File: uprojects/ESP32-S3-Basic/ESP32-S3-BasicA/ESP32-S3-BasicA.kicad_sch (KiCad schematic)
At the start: 5 parts, among them U1 ESP32-S3-WROOM-1x-N8R8

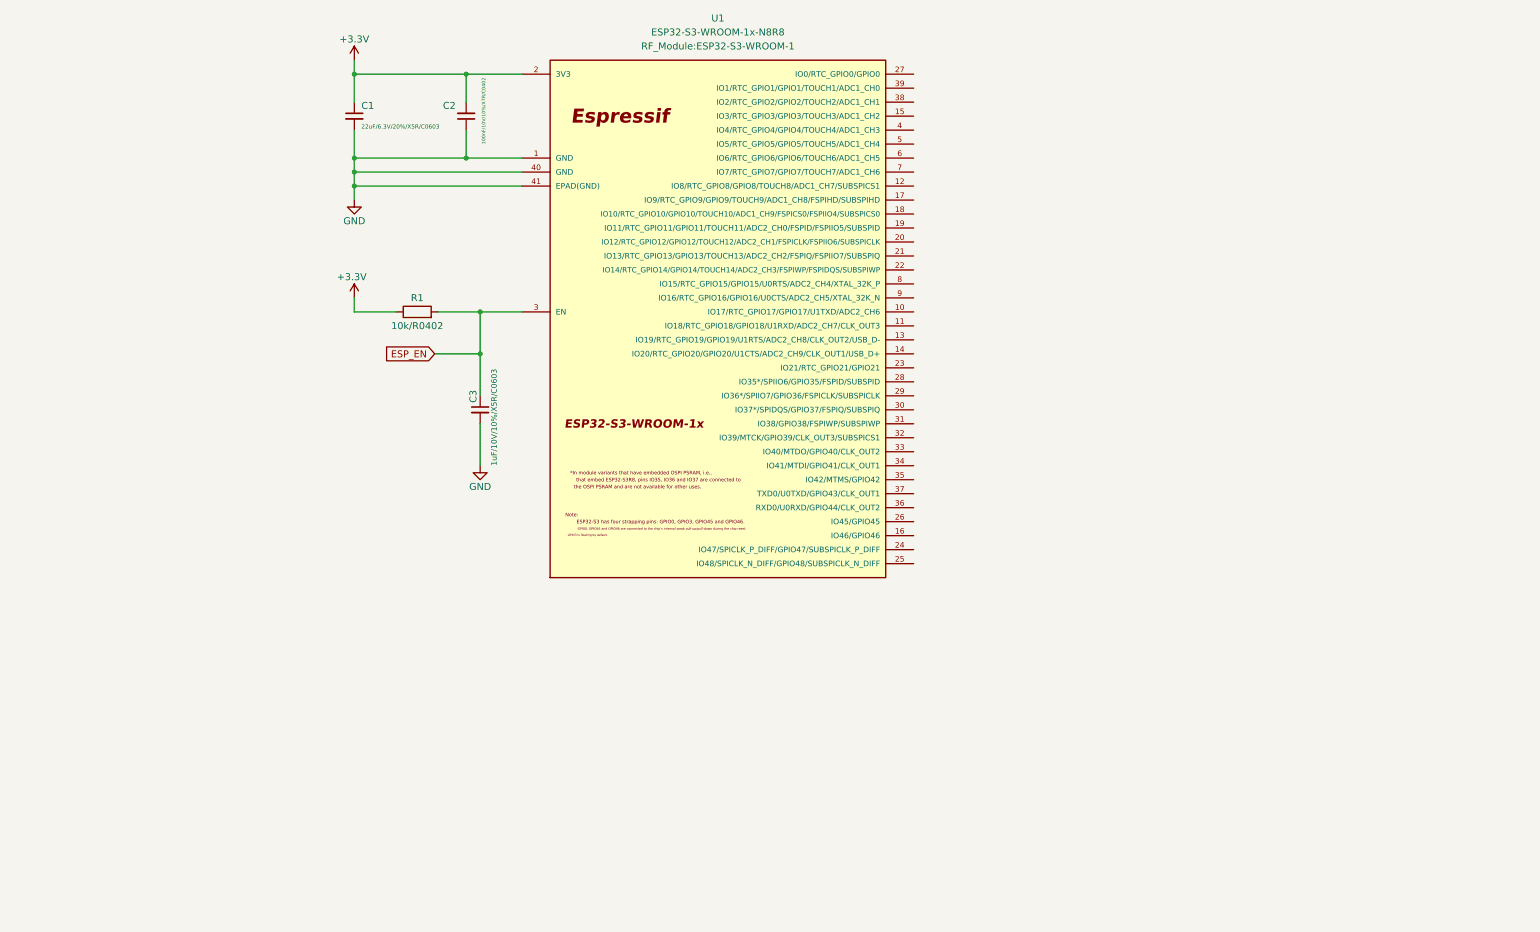
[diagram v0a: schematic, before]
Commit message: April 1 commit
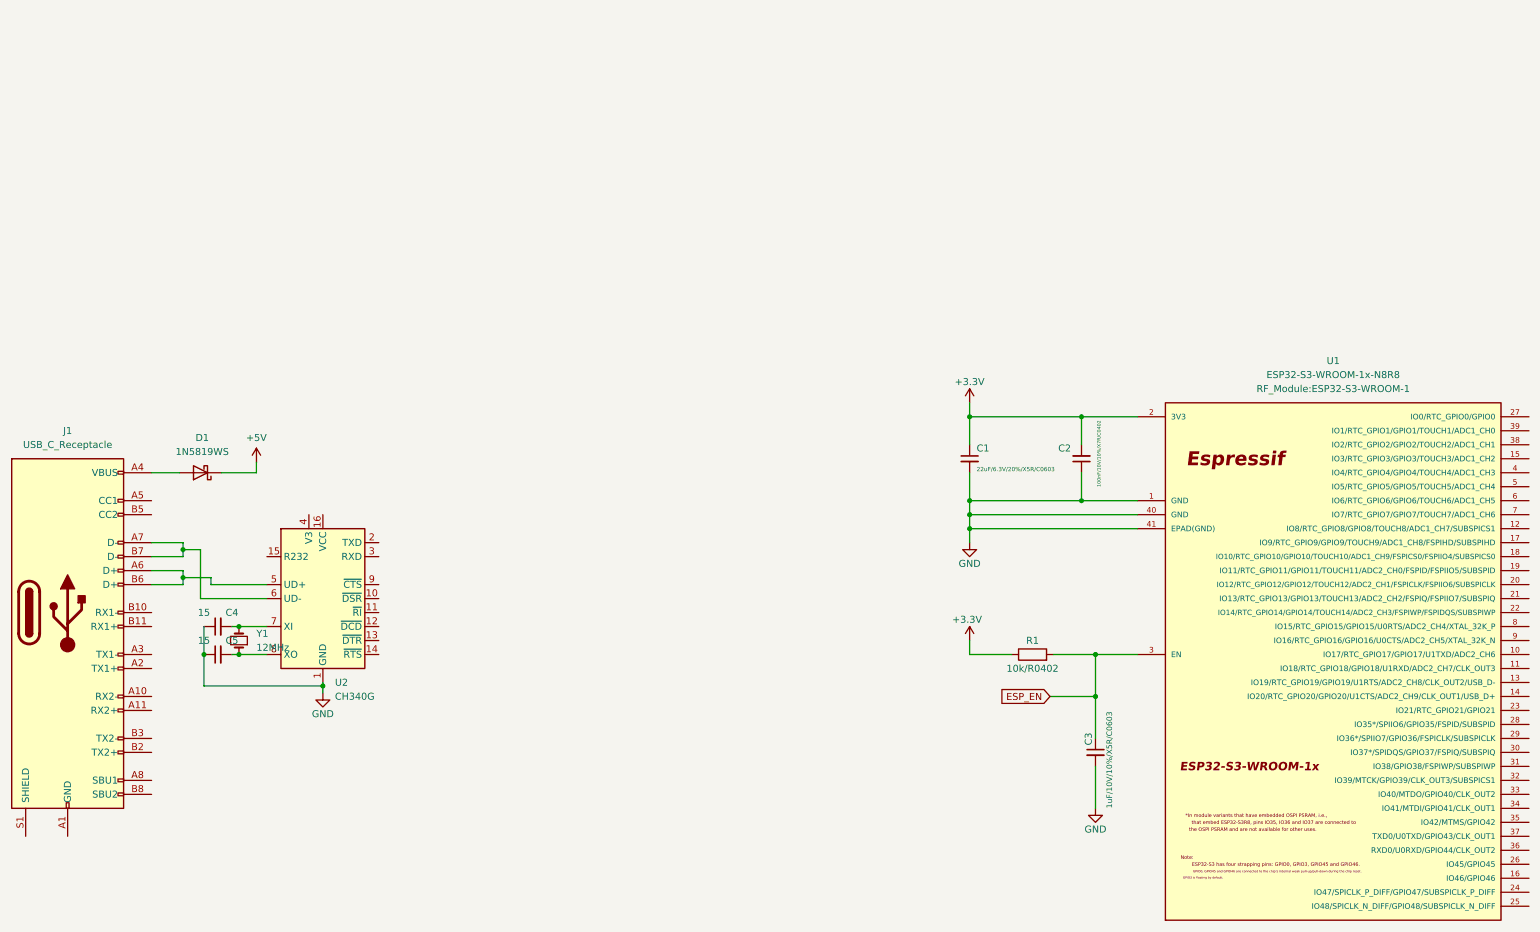
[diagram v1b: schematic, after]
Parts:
- added C4, C5: 15, Capacitor_SMD:C_0805_2012Metric_Pad1.18x1.45mm_HandSolder, symbol Device:C_Small
- added D1: 1N5819WS, Diode_SMD:D_SOD-323, symbol Diode:1N5819WS
- added J1: USB_C_Receptacle, Connector_USB:USB_C_Receptacle_Amphenol_12401610E4-2A_CircularHoles, symbol Connector:USB_C_Receptacle
- added U2: CH340G, Package_SO:SOIC-16_3.9x9.9mm_P1.27mm, symbol Interface_USB:CH340G
- added Y1: 12MHz, Crystal:Crystal_HC49-U_Vertical, symbol Device:Crystal_Small
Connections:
- net GND: now also C4.1, C5.1, U2.1 (GND)
- new net: C5.2, U2.8 (XO), Y1.1
- new net: C4.2, U2.7 (XI), Y1.2
- new net: J1.A1 (GND), J1.A12 (GND), J1.B1 (GND), J1.B12 (GND)
- new net: D1.2 (A), J1.A4 (VBUS), J1.A9 (VBUS), J1.B4 (VBUS), J1.B9 (VBUS)
- new net: J1.A6 (D+), J1.B6 (D+), U2.5 (UD+)
- new net: J1.A7 (D-), J1.B7 (D-), U2.6 (UD-)
- new net +5V: D1.1 (K)
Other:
- moved on the sheet: C1, C2, C3, R1, U1
